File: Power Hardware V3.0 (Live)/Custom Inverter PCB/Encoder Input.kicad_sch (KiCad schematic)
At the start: 12 parts, among them J6 1990041, U6 OP292GSZ-REEL

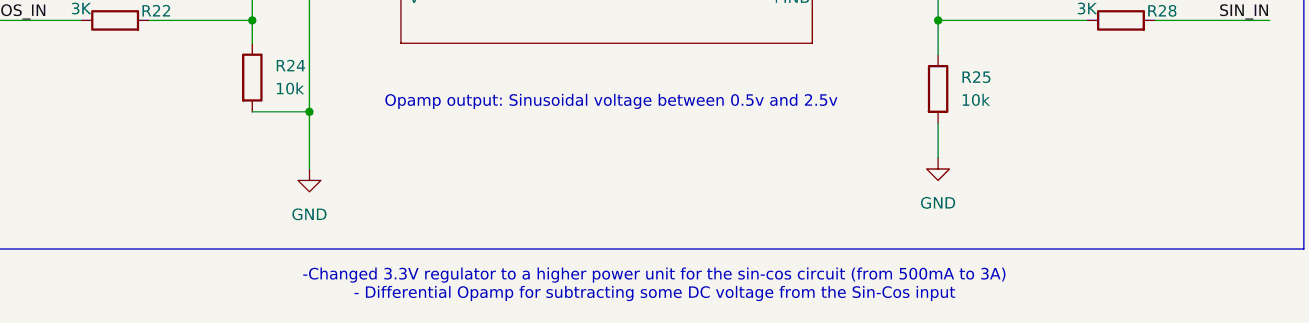
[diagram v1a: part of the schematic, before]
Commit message: V3 push
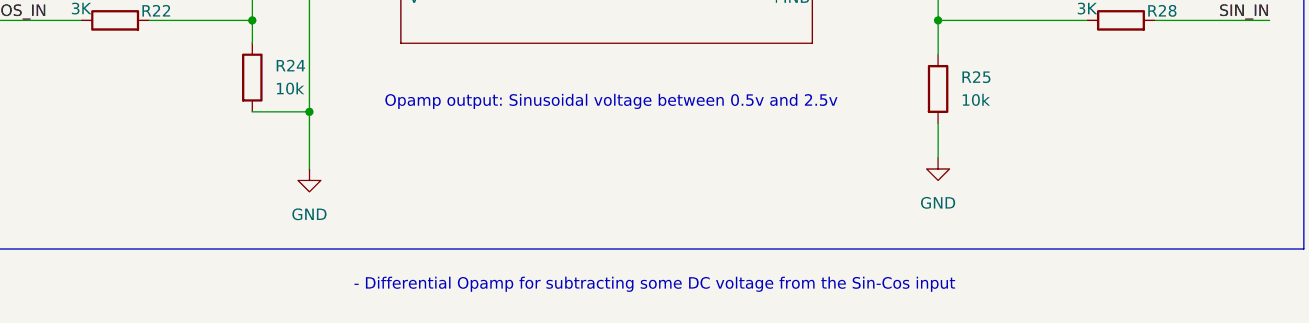
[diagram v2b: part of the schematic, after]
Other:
- note added: "- Differential Opamp for subtracting some DC voltage from the Sin-Cos input"
- note removed: "-Changed 3.3V regulator to a higher power unit for the sin-cos circuit (from 500mA to 3A) - Differential Opamp for subtracting some DC voltage from the Sin-Cos input"
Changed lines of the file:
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@@
 		)
 	)
-	(text "-Changed 3.3V regulator to a higher power unit for the sin-cos circuit (from 500mA to 3A)\n- Differential Opamp for subtracting some DC voltage from the Sin-Cos input\n"
+	(text "- Differential Opamp for subtracting some DC voltage from the Sin-Cos input\n"
 		(exclude_from_sim no)
 		(at 164.084 106.934 0)

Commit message: changes
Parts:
- R21: Part Number (none) -> ERA-6AEB103V
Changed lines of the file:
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@@
+			)
+		)
+		(property "Part Number" "ERA-6AEB103V"
+			(at 99.06 69.85 0)
+			(effects
+				(font
+					(size 1.27 1.27)
+				)
+				(hide yes)
 			)
 		)
